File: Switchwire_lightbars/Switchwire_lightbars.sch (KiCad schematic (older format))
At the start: 3 parts, among them J1 Conn_01x03_Male

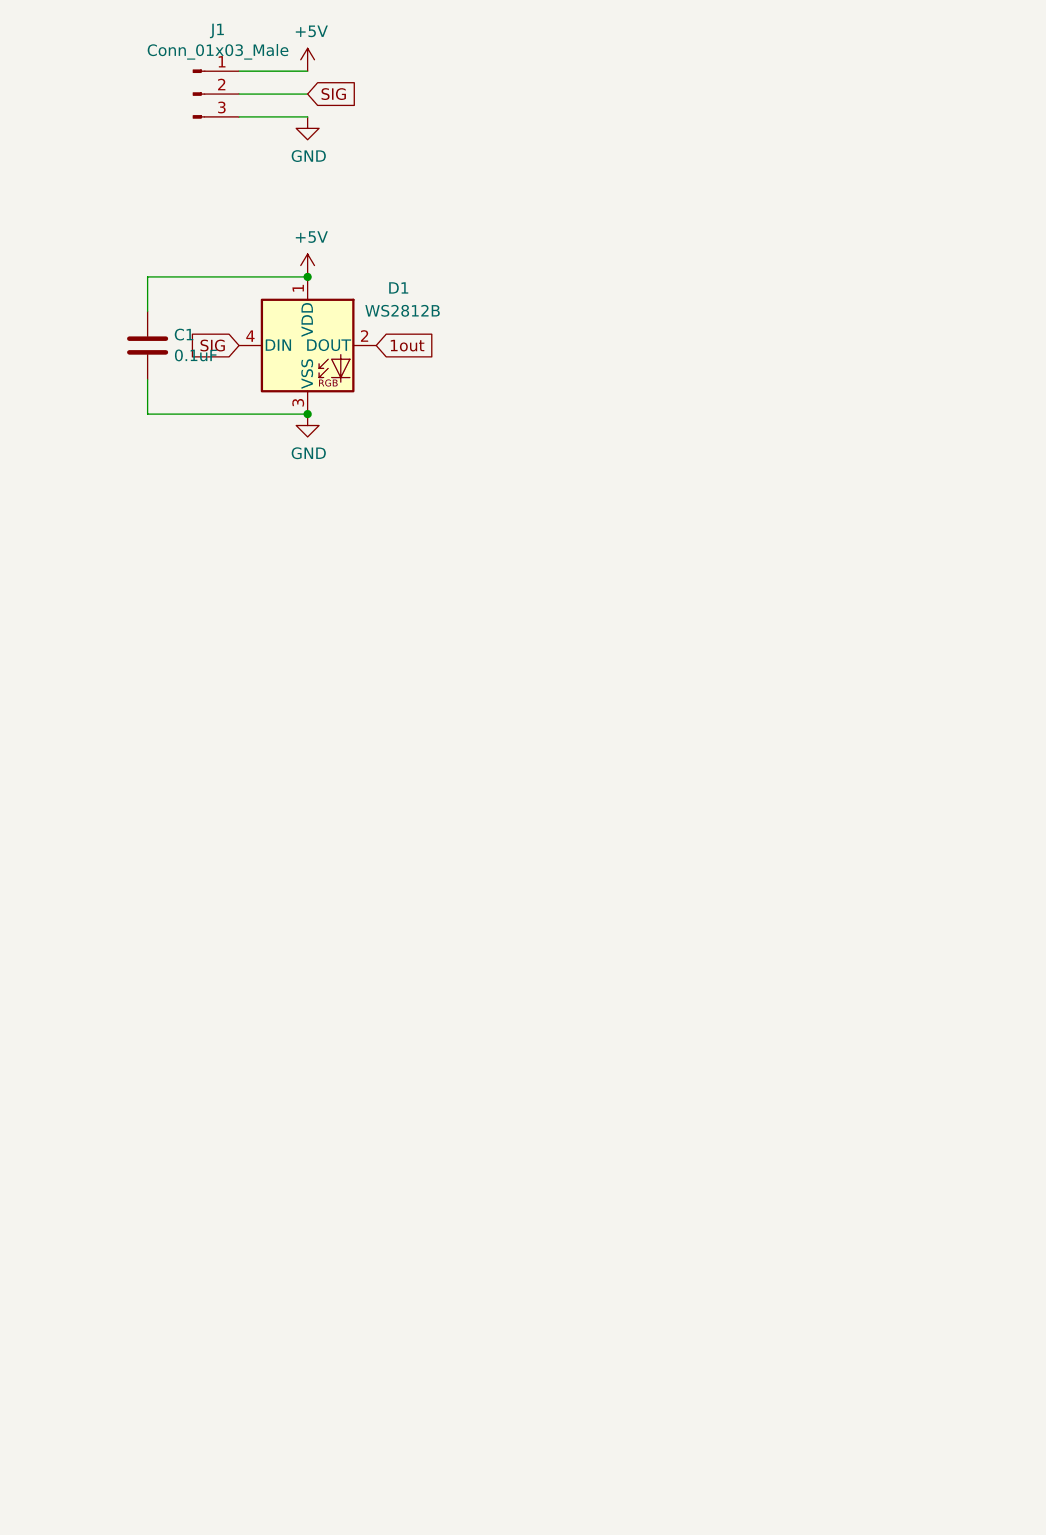
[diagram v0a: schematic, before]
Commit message: Another few changes
Another few changes
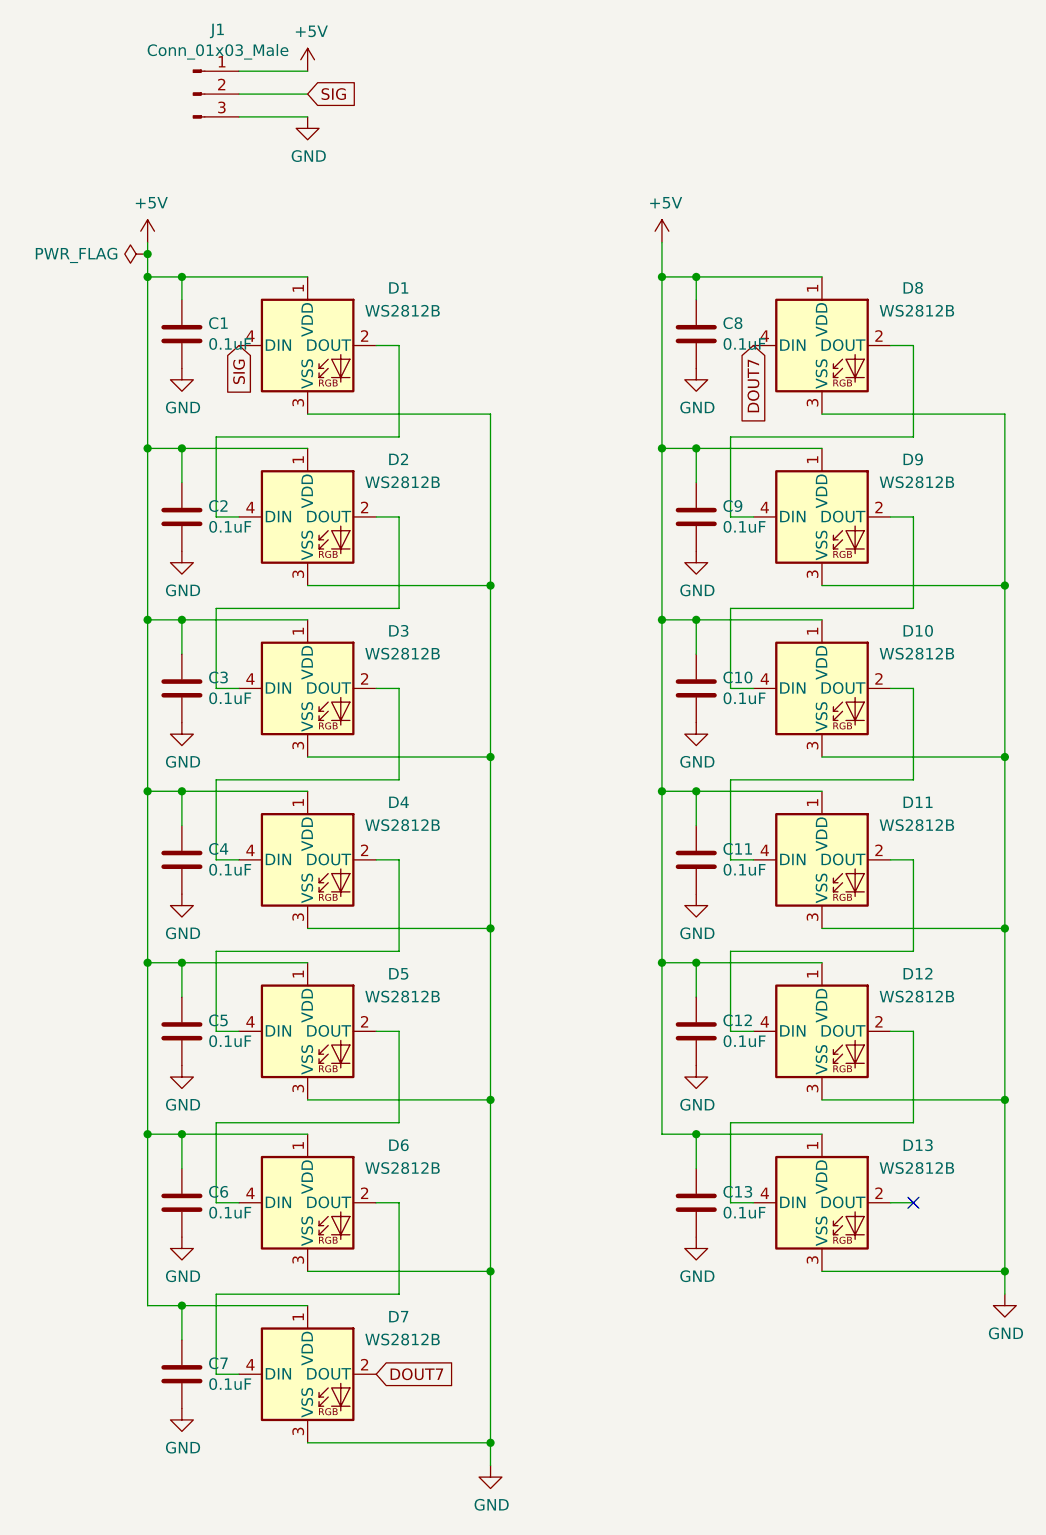
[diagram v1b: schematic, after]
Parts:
- added C10, C11, C12, C13, C2, C3, C4, C5, C6, C7, C8, C9: 0.1uF, Capacitor_SMD:C_0805_2012Metric, symbol Device:C
- added D10, D11, D12, D13, D2, D3, D4, D5, D6, D7, D8, D9: WS2812B, LED_SMD:LED_WS2812B_PLCC4_5.0x5.0mm_P3.2mm, symbol LED:WS2812B
- J1: footprint Connector_JST:JST_XH_S3B-XH-A_1x03_P2.50mm_Horizontal -> Connector_JST:JST_SUR_SM03B-SURS-TF_1x03-1MP_P0.80mm_Horizontal
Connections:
- net +5V: now also C10.1, C11.1, C12.1, C13.1, C2.1, C3.1, C4.1, C5.1, C6.1, C7.1, C8.1, C9.1, D10.1 (VDD), D11.1 (VDD), D12.1 (VDD), D13.1 (VDD), D2.1 (VDD), D3.1 (VDD), D4.1 (VDD), D5.1 (VDD), D6.1 (VDD), D7.1 (VDD), D8.1 (VDD), D9.1 (VDD)
- net GND: now also C10.2, C11.2, C12.2, C13.2, C2.2, C3.2, C4.2, C5.2, C6.2, C7.2, C8.2, C9.2, D10.3 (VSS), D11.3 (VSS), D12.3 (VSS), D13.3 (VSS), D2.3 (VSS), D3.3 (VSS), D4.3 (VSS), D5.3 (VSS), D6.3 (VSS), D7.3 (VSS), D8.3 (VSS), D9.3 (VSS)
- net 1out: no longer names the net of D1.2 (DOUT)
- net 1out: now also D2.4 (DIN)
- new net: D2.2 (DOUT), D3.4 (DIN)
- new net: D3.2 (DOUT), D4.4 (DIN)
- new net: D4.2 (DOUT), D5.4 (DIN)
- new net: D5.2 (DOUT), D6.4 (DIN)
- new net: D6.2 (DOUT), D7.4 (DIN)
- new net: D8.2 (DOUT), D9.4 (DIN)
- new net: D10.4 (DIN), D9.2 (DOUT)
- new net: D10.2 (DOUT), D11.4 (DIN)
- new net: D11.2 (DOUT), D12.4 (DIN)
- new net: D12.2 (DOUT), D13.4 (DIN)
- new net DOUT7: D7.2 (DOUT), D8.4 (DIN)
- no-connect marks 0 -> 1
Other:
- moved on the sheet: C1
